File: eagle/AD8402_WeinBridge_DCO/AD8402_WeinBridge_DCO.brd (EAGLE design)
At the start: 70.8 x 45.7 mm, 28 parts, among them IC1 NJM2732, IC2 AD8402_DIP14, IC3 TLE2426LP

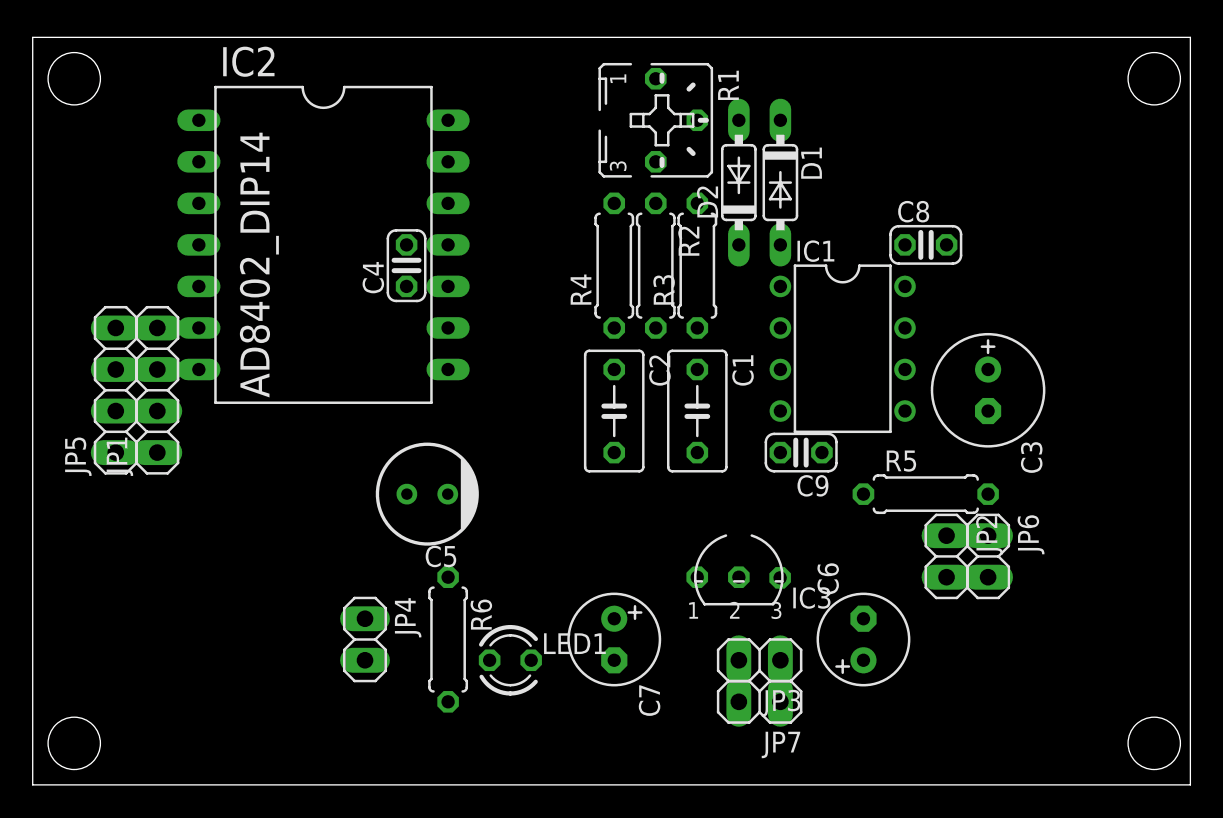
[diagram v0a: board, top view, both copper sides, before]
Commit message: Update eagle files
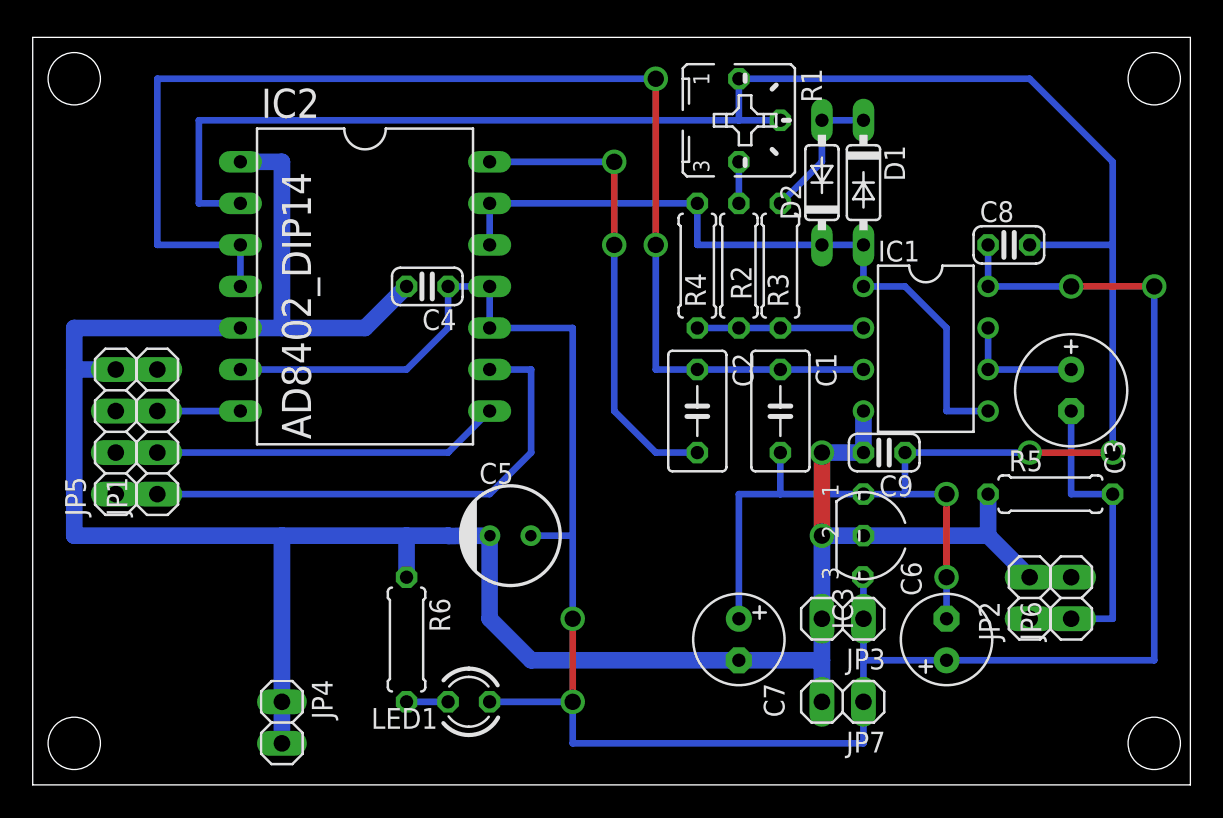
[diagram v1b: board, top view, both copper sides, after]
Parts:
- moved IC3 8.03 mm to (50.8, 15.2), turned to 270 degrees
- moved C7 7.62 mm to (43.2, 8.89)
- moved R5 7.62 mm to (62.2, 17.8)
- moved JP4 7.18 mm to (15.2, 3.81)
- moved C5 5.68 mm to (29.2, 15.2), turned to 0 degrees
- moved JP2 5.68 mm to (61.0, 11.4), turned to 90 degrees
- moved JP6 5.68 mm to (63.5, 11.4), turned to 90 degrees
- moved JP3 5.68 mm to (49.5, 10.2)
- moved C6 5.08 mm to (55.9, 8.89)
- moved C1 5.08 mm to (45.7, 22.9)
- moved C2 5.08 mm to (40.6, 22.9)
- moved C3 5.08 mm to (63.5, 24.1)
- moved C8 5.08 mm to (59.7, 33.0)
- moved C9 5.08 mm to (52.1, 20.3)
- moved D1 5.08 mm to (50.8, 36.8)
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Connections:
- removed net N$7: LED1.A, R6.1
- new net N$3: LED1.K, R6.2
- net +5V: now also LED1.A; no longer R6.2
- net GND: now also R6.1; no longer LED1.K
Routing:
- net GND: track 0.00 -> 158.1 mm, vias 0 -> 2
- net +5V: track 0.00 -> 140.8 mm, vias 0 -> 4
- net VCC/2: track 0.00 -> 139.3 mm, vias 0 -> 4
- net N$10: track 0.00 -> 78.7 mm, vias 0 -> 2
- net N$6: track 0.00 -> 44.2 mm
- net SCK: track 0.00 -> 34.1 mm
- net N$11: track 0.00 -> 29.0 mm, vias 0 -> 2
- net MOSI: track 0.00 -> 23.9 mm
- net N$4: track 0.00 -> 20.3 mm
- net N$1: track 0.00 -> 10.2 mm
- net N$5: track 0.00 -> 8.67 mm
- net N$12: track 0.00 -> 7.62 mm
- net CS: track 0.00 -> 7.62 mm
- net N$3: track 0.00 -> 2.54 mm
- net N$2: track 0.00 -> 2.54 mm
